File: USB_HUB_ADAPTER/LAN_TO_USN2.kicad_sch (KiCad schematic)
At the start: 26 parts, among them J6 RJ_45_CONN_100G_J1B1211CCD, U6 LAN9500AI-ABZJ-TR, Y3 25MHz

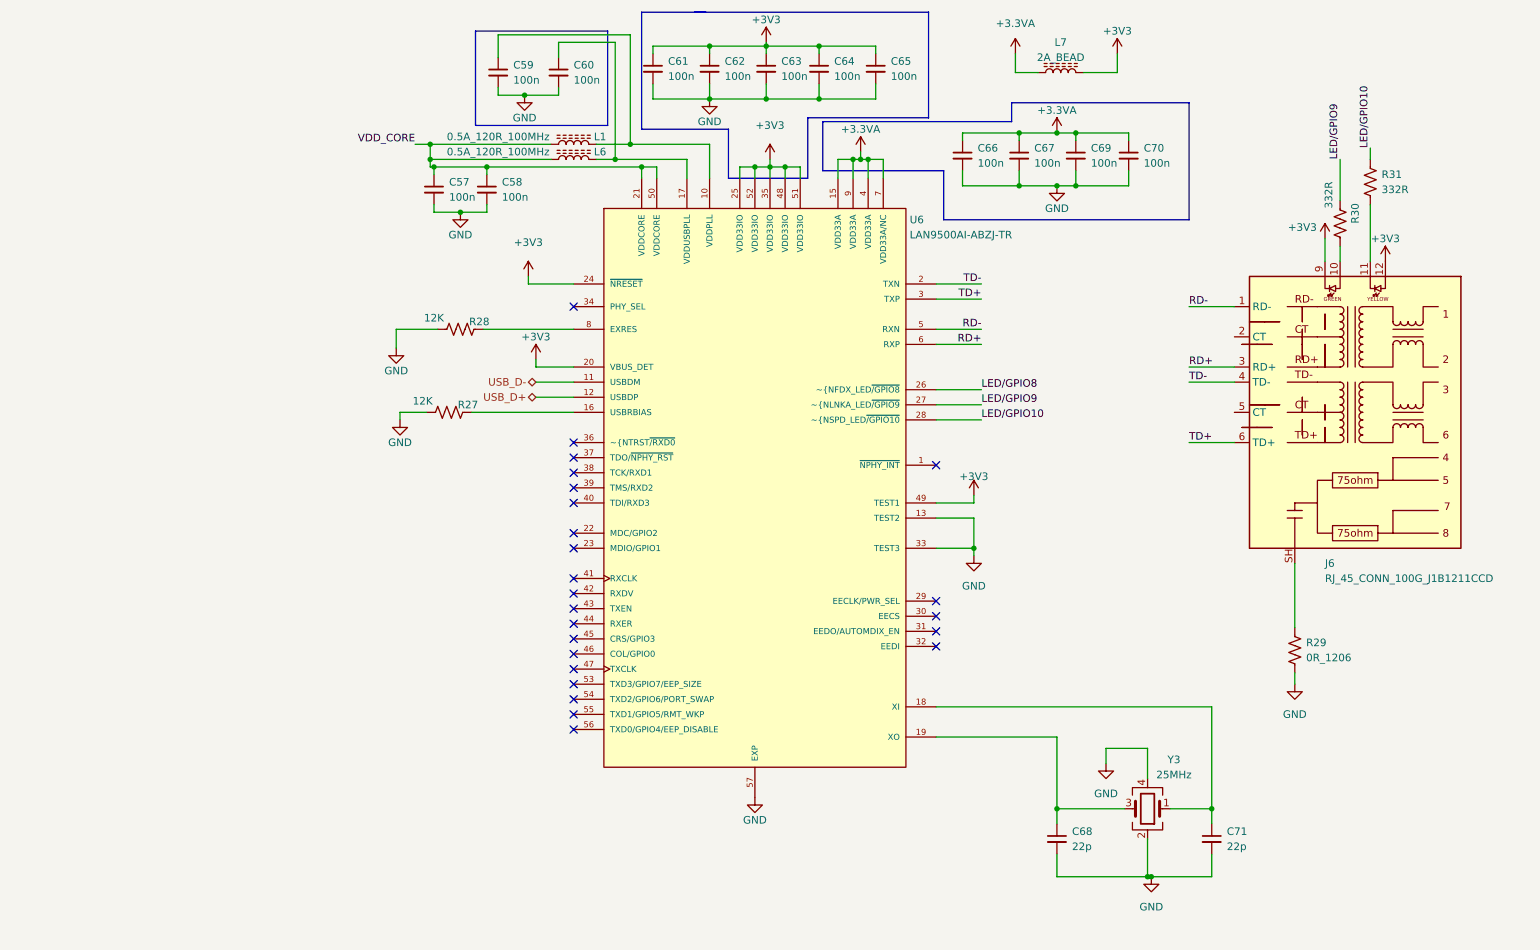
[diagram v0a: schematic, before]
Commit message: v2 layout update
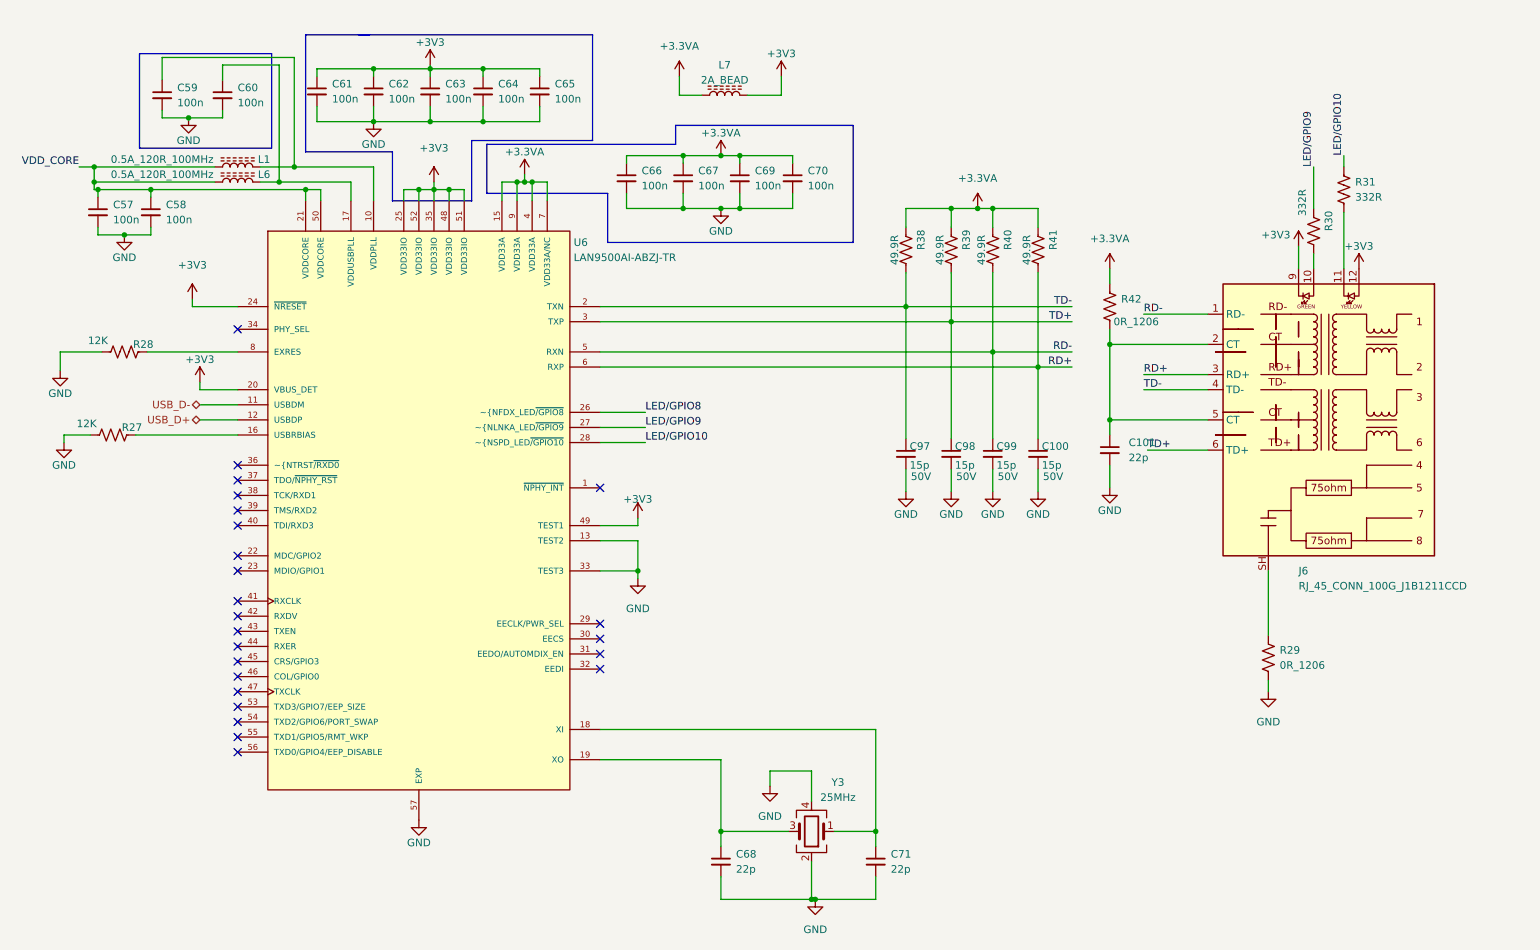
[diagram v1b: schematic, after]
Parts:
- added C100, C97, C98, C99: 15p, Capacitor_SMD:C_0402_1005Metric, symbol Device:C_Small
- added C101: 22p, Capacitor_SMD:C_0805_2012Metric, symbol Device:C_Small
- added R38, R39, R40, R41: 49.9R, Resistor_SMD:R_0402_1005Metric, symbol Device:R_US
- added R42: 0R_1206, Resistor_SMD:R_1206_3216Metric, symbol Device:R_US
- C57, C58, C59, C60, C61, C62, C63, C64, C65, C66, C67, C68, C69, C70, C71: footprint (none) -> Capacitor_SMD:C_0402_1005Metric
- L1, L6, L7: footprint (none) -> Inductor_SMD:L_0402_1005Metric
- R27, R28, R30, R31: footprint (none) -> Resistor_SMD:R_0402_1005Metric
- R29: footprint (none) -> Resistor_SMD:R_1206_3216Metric
- U6: footprint QFN50P800X800X100-57N -> greencharge-footprints:LAN950X_QFN50P800X800X100-57N
- Y3: footprint (none) -> Crystal:Crystal_SMD_2520-4Pin_2.5x2.0mm
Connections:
- net +3.3VA: now also R38.2, R39.2, R40.2, R41.2, R42.1
- net GND: now also C100.2, C101.2, C97.2, C98.2, C99.2
- net RD+: now also C100.1, R41.1
- net RD-: now also C99.1, R40.1
- net TD+: now also C98.1, R39.1
- net TD-: now also C97.1, R38.1
- net at J6.2 (CT): now also J6.5 (CT), C101.1, R42.2
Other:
- moved on the sheet: C57, C58, C59, C60, C61, C62, C63, C64, C65, C66, C67, C68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
